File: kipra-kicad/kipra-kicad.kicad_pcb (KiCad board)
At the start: 2 copper layers, 128.2 x 134.8 mm, 52 parts

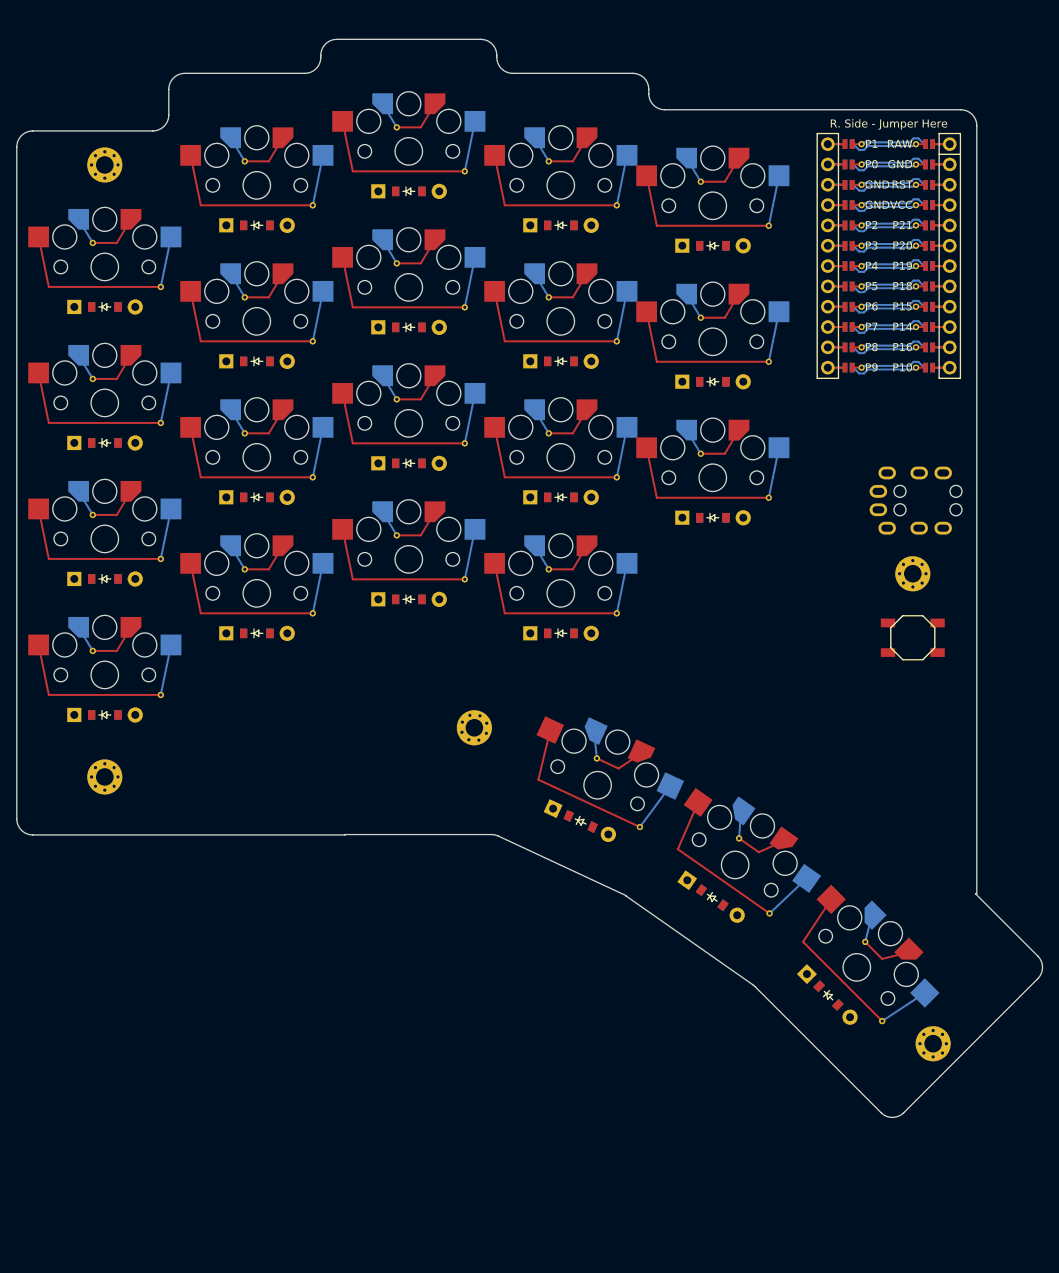
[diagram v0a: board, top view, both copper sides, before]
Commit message: checkpoint before starting over to move row pins down one slot to the corner
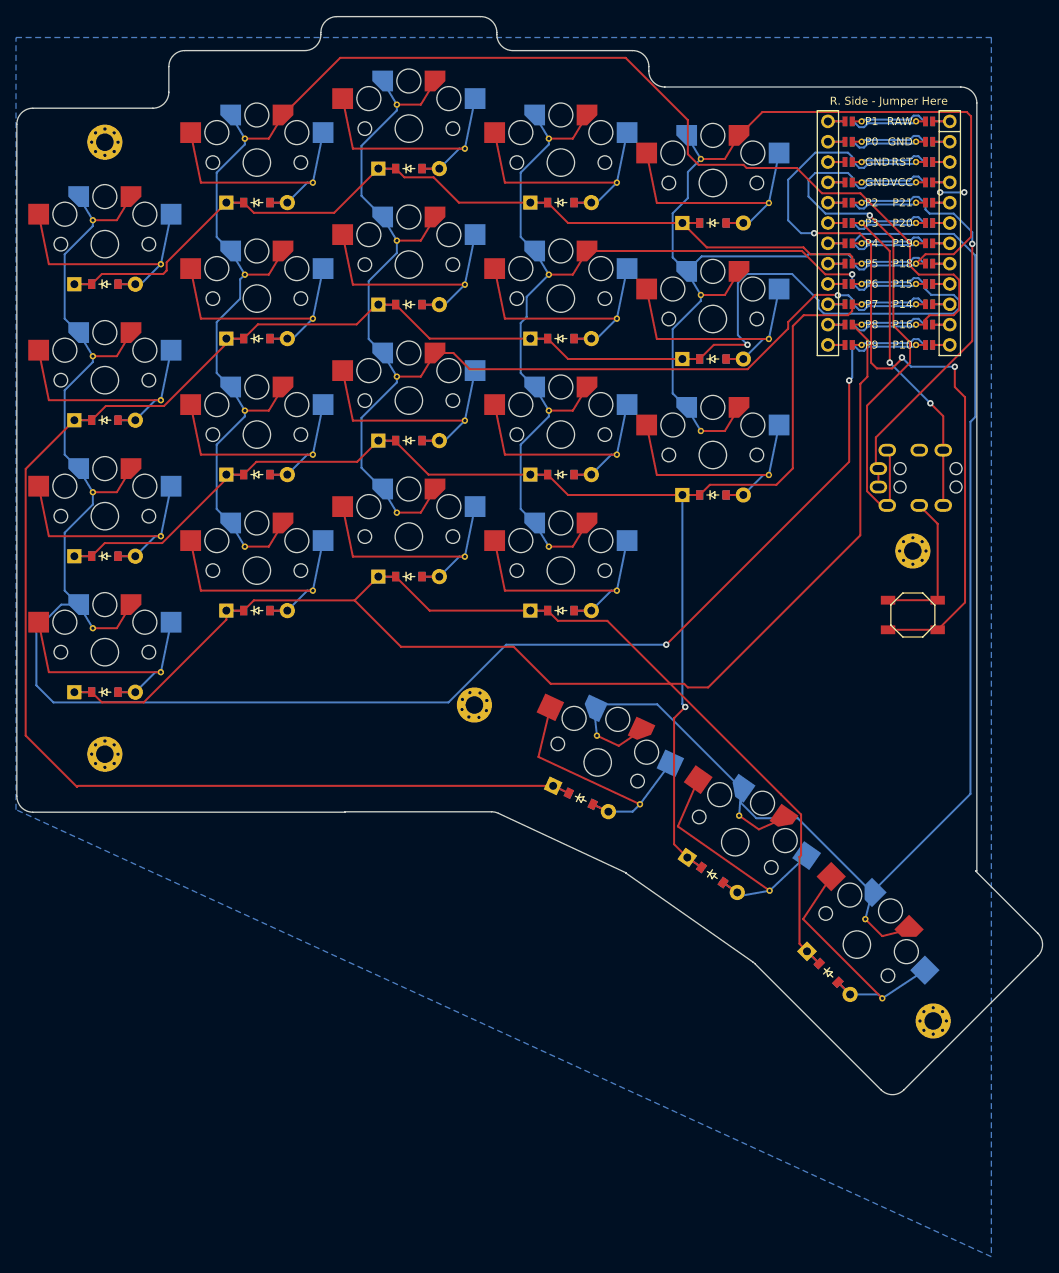
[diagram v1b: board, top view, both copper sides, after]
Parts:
- moved D11 2.84 mm to (138.0, 53.7)
- moved TRRS1 2.84 mm to (208.0, 76.5)
- moved D21 2.84 mm to (175.9, 125.0)
- moved S21 2.84 mm to (178.8, 120.9)
- moved D12 2.84 mm to (138.0, 36.7)
- moved D16 2.84 mm to (157.0, 41.0)
- moved S20 2.84 mm to (194.0, 133.7)
- moved S3 2.84 mm to (100.0, 63.2)
- moved D17 2.84 mm to (176.0, 77.5)
- moved S18 2.84 mm to (176.0, 55.5)
- moved S17 2.84 mm to (176.0, 72.5)
- moved D14 2.84 mm to (157.0, 75.0)
- moved D2 2.84 mm to (100.0, 85.2)
- moved S19 2.84 mm to (176.0, 38.5)
- moved _1 2.84 mm to (100.0, 109.9)
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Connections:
- MCU1 pad 1: RAW -> MCU1_1
- MCU1 pad 10: P14 -> MCU1_10
- MCU1 pad 11: P16 -> MCU1_11
- MCU1 pad 12: P10 -> MCU1_12
- MCU1 pad 2: GND -> MCU1_2
- MCU1 pad 3: RST -> MCU1_3
- MCU1 pad 4: VCC -> MCU1_4
- MCU1 pad 5: P21 -> MCU1_5
- MCU1 pad 6: P20 -> MCU1_6
- MCU1 pad 7: P19 -> MCU1_7
- MCU1 pad 8: P18 -> MCU1_8
- MCU1 pad 9: P15 -> MCU1_9
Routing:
- net (no net): track 806.3 -> 0.00 mm
- net P6: track 0.00 -> 274.8 mm, vias 0 -> 1
- net P8: track 0.00 -> 253.8 mm
- net P10: track 14.2 -> 240.8 mm, vias 0 -> 2
- net P16: track 0.00 -> 209.8 mm
- net P7: track 0.00 -> 198.4 mm, vias 0 -> 1
- net P19: track 0.00 -> 186.6 mm
- net P14: track 0.00 -> 157.3 mm, vias 0 -> 1
- net P18: track 0.00 -> 147.6 mm
- net P15: track 0.00 -> 133.1 mm, vias 0 -> 1
- net P5: track 0.00 -> 132.6 mm
- net RST: track 0.00 -> 103.9 mm, vias 0 -> 3
- net VCC: track 0.00 -> 75.9 mm, vias 0 -> 1
- net index_four: track 101.6 -> 35.3 mm
- net pinky_one: track 101.4 -> 35.3 mm
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- added copper zone on B.Cu, net GND
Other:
- outline, holes or cut-outs redrawn
- net class Default removed
- board text added: "P2"
